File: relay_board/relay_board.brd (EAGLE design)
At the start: 42.1 x 49.3 mm, 40 parts, among them IC1 PIC16F1825DIL14, IC2 6N138, IC3 78L05Z

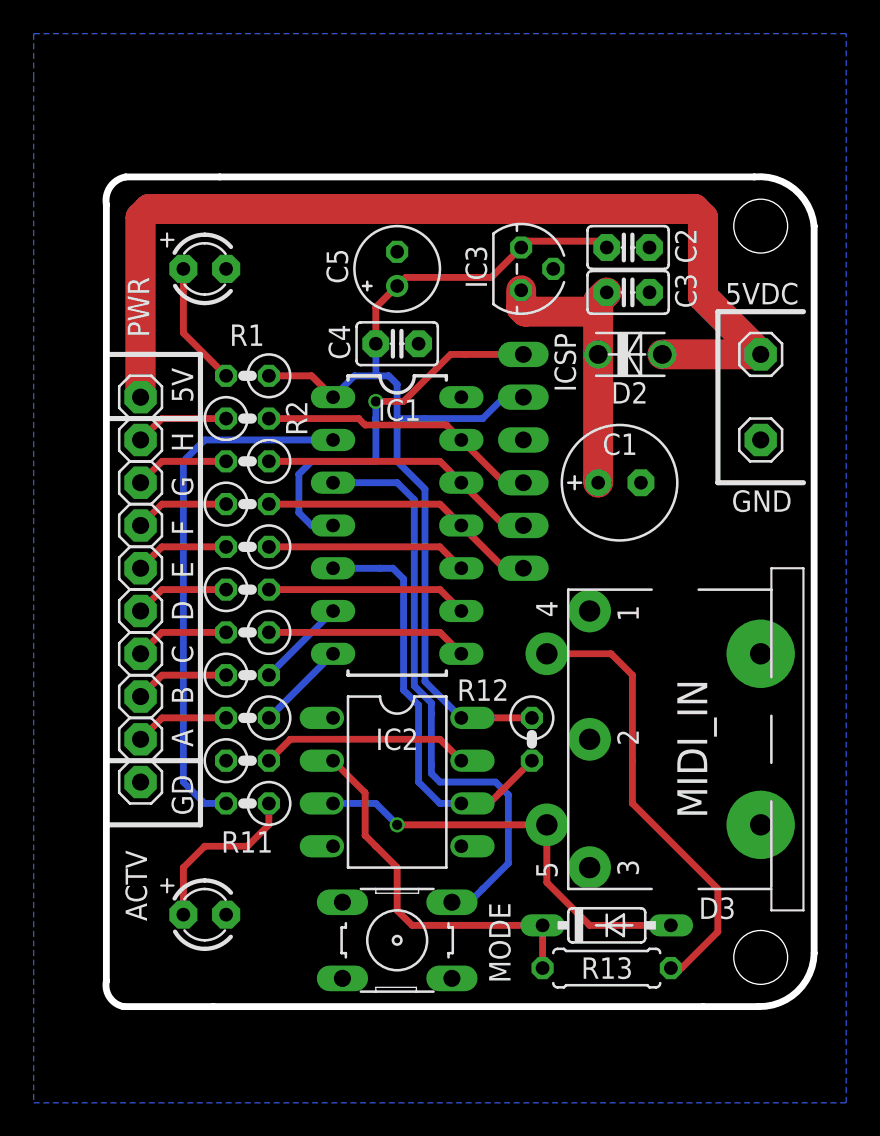
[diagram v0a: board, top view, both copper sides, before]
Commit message: working on relay board
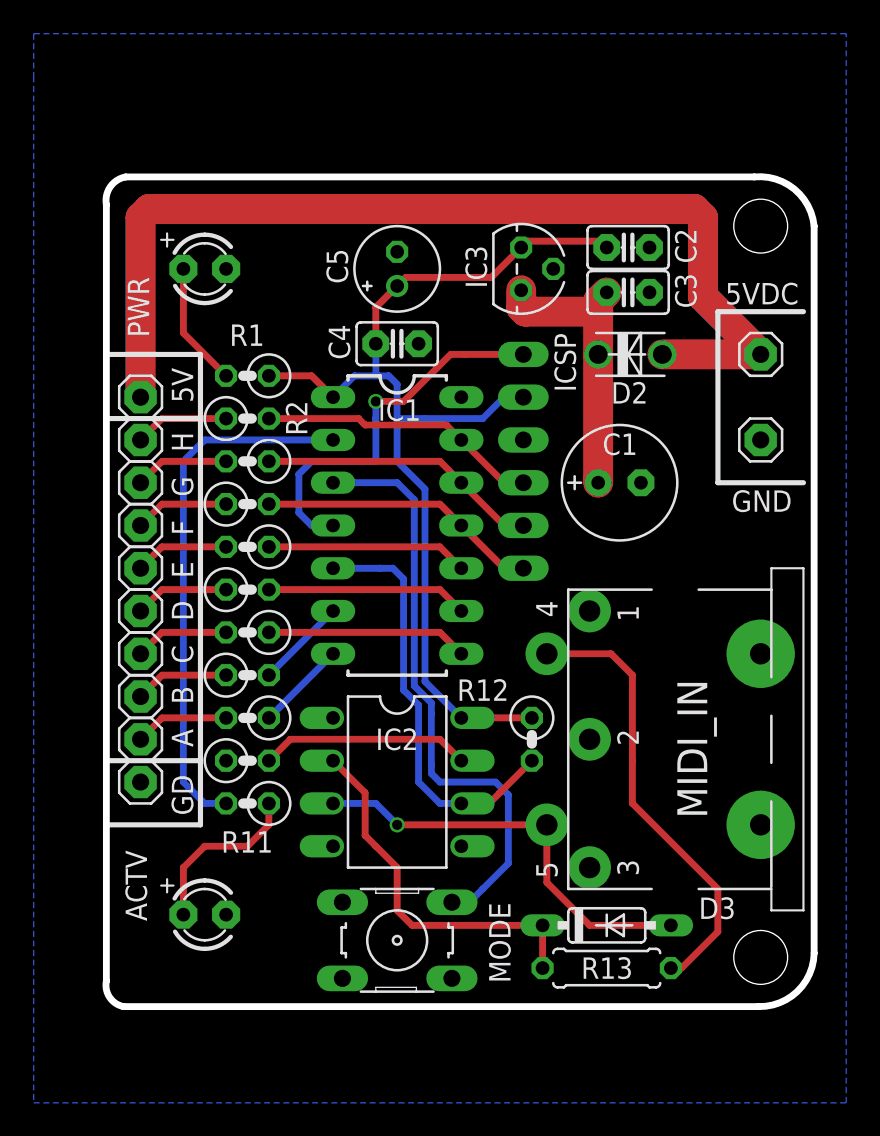
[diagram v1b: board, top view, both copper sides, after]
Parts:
- R1, R11: value (none) -> 1k
- R10, R12: value (none) -> 1k5
- R13: value (none) -> 220
- R2, R3, R4, R5, R6, R7, R8, R9: value (none) -> 100r
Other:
- outline, holes or cut-outs redrawn
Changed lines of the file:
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@@
 <?xml version="1.0" encoding="utf-8"?>
 <!DOCTYPE eagle SYSTEM "eagle.dtd">
-<eagle version="6.4">
+<eagle version="6.6.0">
 <drawing>
 <settings>
@@
 <plain>
 <wire x1="59.055" y1="34.29" x2="59.055" y2="77.47" width="0.4064" layer="20"/>
-<wire x1="23.368" y1="31.115" x2="52.451" y2="31.115" width="0.4064" layer="20"/>
-<wire x1="52.451" y1="31.115" x2="55.753" y2="31.115" width="0.4064" layer="20"/>
+<wire x1="18.034" y1="31.115" x2="55.753" y2="31.115" width="0.4064" layer="20"/>
 <wire x1="55.753" y1="31.115" x2="59.055" y2="34.29" width="0.4064" layer="20" curve="90"/>
 <wire x1="59.055" y1="77.47" x2="55.499" y2="80.391" width="0.4064" layer="20" curve="90"/>
-<wire x1="23.749" y1="80.391" x2="55.499" y2="80.391" width="0.4064" layer="20"/>
+<wire x1="18.161" y1="80.391" x2="55.499" y2="80.391" width="0.4064" layer="20"/>
 <hole x="55.88" y="77.47" drill="3.2"/>
 <hole x="55.88" y="34.036" drill="3.2"/>
@@
 <wire x1="53.34" y1="72.39" x2="53.34" y2="62.23" width="0.3048" layer="21"/>
 <wire x1="53.34" y1="62.23" x2="58.42" y2="62.23" width="0.3048" layer="21"/>
-<wire x1="23.749" y1="80.391" x2="18.161" y2="80.391" width="0.4064" layer="20"/>
 <wire x1="18.161" y1="80.391" x2="17.018" y2="78.74" width="0.4064" layer="20" curve="90"/>
 <wire x1="17.018" y1="78.74" x2="17.018" y2="32.639" width="0.4064" layer="20"/>
 <wire x1="17.018" y1="32.639" x2="18.034" y2="31.115" width="0.4064" layer="20" curve="90"/>
-<wire x1="18.034" y1="31.115" x2="23.368" y2="31.115" width="0.4064" layer="20"/>
 <wire x1="17.018" y1="69.85" x2="22.606" y2="69.85" width="0.3048" layer="21"/>
 <wire x1="22.606" y1="69.85" x2="22.606" y2="66.04" width="0.3048" layer="21"/>
 <wire x1="22.606" y1="66.04" x2="22.606" y2="45.72" width="0.3048" layer="21"/>
-<wire x1="22.606" y1="45.72" x2="22.606" y2="42.291" width="0.3048" layer="21"/>
+<wire x1="22.606" y1="45.72" x2="22.606" y2="41.91" width="0.3048" layer="21"/>
 <wire x1="17.018" y1="41.91" x2="22.606" y2="41.91" width="0.3048" layer="21"/>
-<wire x1="22.606" y1="41.91" x2="22.606" y2="42.291" width="0.3048" layer="21"/>
 <wire x1="17.018" y1="45.72" x2="22.606" y2="45.72" width="0.3048" layer="21"/>
 <wire x1="17.018" y1="66.04" x2="22.606" y2="66.04" width="0.3048" layer="21"/>
@@
 <attribute name="NAME" x="52.705" y="42.291" size="1.778" layer="25" ratio="10" rot="R90"/>
 </element>
-<element name="R13" library="rcl" package="0207/7" value="" x="46.736" y="33.401" smashed="yes">
+<element name="R13" library="rcl" package="0207/7" value="220" x="46.736" y="33.401" smashed="yes">
 <attribute name="NAME" x="45.212" y="32.766" size="1.27" layer="25"/>
-<attribute name="VALUE" x="46.101" y="30.861" size="1.27" layer="27"/>
-</element>
-<element name="R10" library="rcl" package="0207/2V" value="" x="25.4" y="45.72" smashed="yes">
-<attribute name="VALUE" x="24.765" y="43.18" size="1.27" layer="27"/>
-</element>
-<element name="R12" library="rcl" package="0207/2V" value="" x="42.291" y="46.99" smashed="yes" rot="R270">
+</element>
+<element name="R10" library="rcl" package="0207/2V" value="1k5" x="25.4" y="45.72" smashed="yes"/>
+<element name="R12" library="rcl" package="0207/2V" value="1k5" x="42.291" y="46.99" smashed="yes" rot="R270">
 <attribute name="NAME" x="37.846" y="49.276" size="1.27" layer="25"/>
-<attribute name="VALUE" x="39.751" y="47.625" size="1.27" layer="27" rot="R270"/>
 </element>
 <element name="C2" library="capacitor-wima" package="C2.5-2" value="" x="48.006" y="76.2" smashed="yes">
@@
 <attribute name="VALUE" x="46.736" y="73.66" size="1.27" layer="27"/>
 </element>
-<element name="R5" library="rcl" package="0207/2V" value="" x="25.4" y="58.42" smashed="yes" rot="R180">
-<attribute name="VALUE" x="26.035" y="60.96" size="1.27" layer="27" rot="R180"/>
-</element>
-<element name="R4" library="rcl" package="0207/2V" value="" x="25.4" y="60.96" smashed="yes">
-<attribute name="VALUE" x="24.765" y="58.42" size="1.27" layer="27"/>
-</element>
-<element name="R3" library="rcl" package="0207/2V" value="" x="25.4" y="63.5" smashed="yes" rot="R180">
-<attribute name="VALUE" x="26.035" y="66.04" size="1.27" layer="27" rot="R180"/>
-</element>
-<element name="R2" library="rcl" package="0207/2V" value="" x="25.4" y="66.04" smashed="yes">
+<element name="R5" library="rcl" package="0207/2V" value="100r" x="25.4" y="58.42" smashed="yes" rot="R180"/>
+<element name="R4" library="rcl" package="0207/2V" value="100r" x="25.4" y="60.96" smashed="yes"/>
+<element name="R3" library="rcl" package="0207/2V" value="100r" x="25.4" y="63.5" smashed="yes" rot="R180"/>
+<element name="R2" library="rcl" package="0207/2V" value="100r" x="25.4" y="66.04" smashed="yes">
 <attribute name="NAME" x="28.956" y="65.024" size="1.27" layer="25" rot="R90"/>
-<attribute name="VALUE" x="24.765" y="63.5" size="1.27" layer="27"/>
-</element>
-<element name="R7" library="rcl" package="0207/2V" value="" x="25.4" y="53.34" smashed="yes" rot="R180">
-<attribute name="VALUE" x="26.035" y="55.88" size="1.27" layer="27" rot="R180"/>
-</element>
-<element name="R9" library="rcl" package="0207/2V" value="" x="25.4" y="48.26" smashed="yes" rot="R180">
-<attribute name="VALUE" x="26.035" y="50.8" size="1.27" layer="27" rot="R180"/>
-</element>
-<element name="R6" library="rcl" package="0207/2V" value="" x="25.4" y="55.88" smashed="yes">
-<attribute name="VALUE" x="24.765" y="53.34" size="1.27" layer="27"/>
-</element>
-<element name="R8" library="rcl" package="0207/2V" value="" x="25.4" y="50.8" smashed="yes">
-<attribute name="VALUE" x="24.765" y="48.26" size="1.27" layer="27"/>
-</element>
+</element>
+<element name="R7" library="rcl" package="0207/2V" value="100r" x="25.4" y="53.34" smashed="yes" rot="R180"/>
+<element name="R9" library="rcl" package="0207/2V" value="100r" x="25.4" y="48.26" smashed="yes" rot="R180"/>
+<element name="R6" library="rcl" package="0207/2V" value="100r" x="25.4" y="55.88" smashed="yes"/>
+<element name="R8" library="rcl" package="0207/2V" value="100r" x="25.4" y="50.8" smashed="yes"/>
 <element name="ICSP" library="microbuilder" package="1X06_OVAL" value="" x="41.783" y="63.5" smashed="yes" rot="R270">
 <attribute name="NAME" x="44.9072" y="67.6148" size="1.27" layer="25" ratio="10" rot="R90"/>
@@
 <attribute name="VALUE" x="24.765" y="73.279" size="1.27" layer="27" ratio="10"/>
 </element>
-<element name="R1" library="rcl" package="0207/2V" value="" x="25.4" y="68.58" smashed="yes" rot="R180">
+<element name="R1" library="rcl" package="0207/2V" value="1k" x="25.4" y="68.58" smashed="yes" rot="R180">
 <attribute name="NAME" x="26.416" y="71.628" size="1.27" layer="25" rot="R180"/>
-<attribute name="VALUE" x="26.035" y="71.12" size="1.27" layer="27" rot="R180"/>
 </element>
 <element name="ACTV" library="adafruit" package="LED3MM" value="" x="22.86" y="36.576" smashed="yes">
@@
 <attribute name="VALUE" x="24.765" y="34.925" size="1.27" layer="27" ratio="10"/>
 </element>
-<element name="R11" library="rcl" package="0207/2V" value="" x="25.4" y="43.18" smashed="yes" rot="R180">
+<element name="R11" library="rcl" package="0207/2V" value="1k" x="25.4" y="43.18" smashed="yes" rot="R180">
 <attribute name="NAME" x="26.924" y="41.529" size="1.27" layer="25" rot="R180"/>
-<attribute name="VALUE" x="26.035" y="45.72" size="1.27" layer="27" rot="R180"/>
 </element>
 <element name="MODE" library="switch-omron" package="B3F-10XX" value="" x="34.29" y="35.052" smashed="yes">
